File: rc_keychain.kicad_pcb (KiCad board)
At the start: 4 copper layers, 63 x 18 mm, 139 parts, among them J2 TYPE-C 16PIN 2MD(073), J3 Touch_Surface_Top, J4 Touch_Surface_Bottom, J5 5034801200, Q1 2N7002T, SW1 TS35CA, U1 SF32LB525UC6, U10 LIS3DH, U12 SN74AUP1G17, U13 ST25R3916B-AQET, U2 GD25Q256EWIGR, U3 TPS25200DRVT, U4 USBLC6-2P6, U5 USBLC6-2P6, U6 CAP1208-1-A4-TR, U7 CAP1208-1-A4-TR, U8 DRV2603RUNT, U9 TPS61040DBV, Y1 48MHz, Y2 32.768khz, Y3 27.12MHz

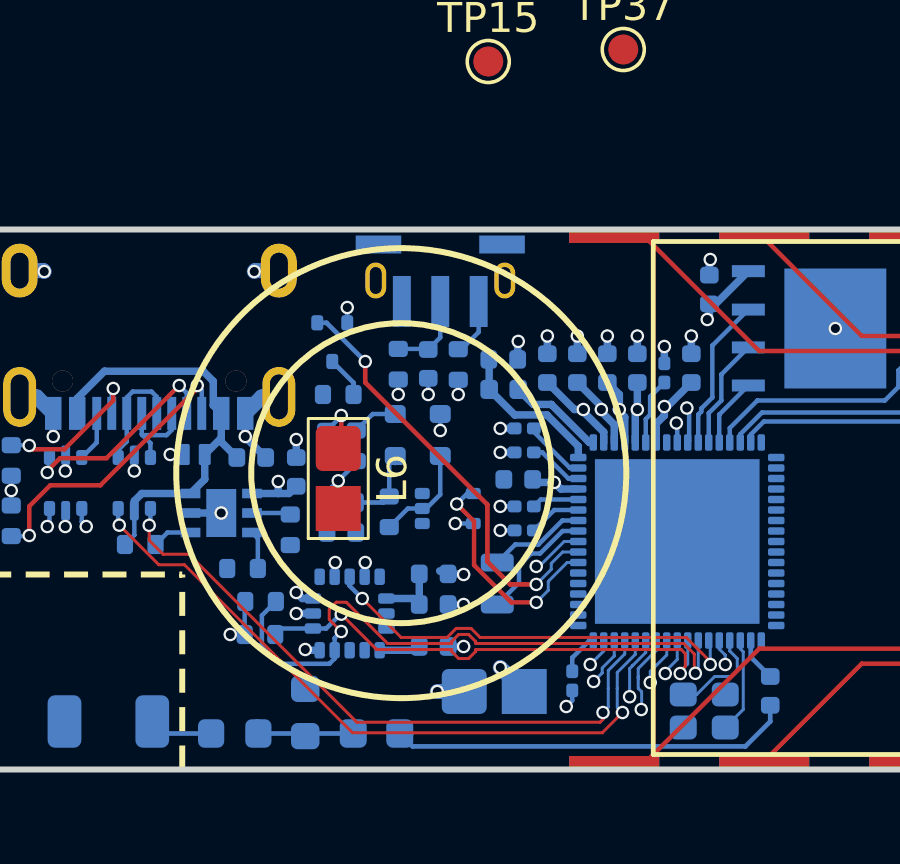
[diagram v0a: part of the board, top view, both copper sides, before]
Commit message: progress before stepping
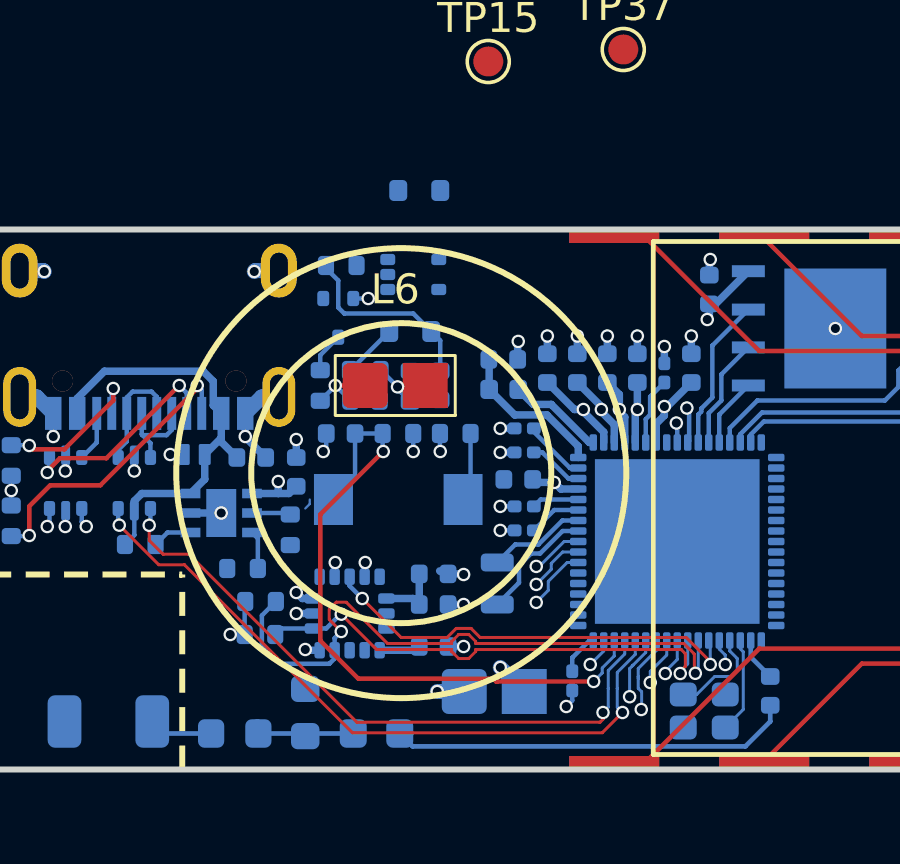
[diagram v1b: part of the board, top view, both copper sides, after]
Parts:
- SW1: value TS35CA -> HX 3X4X2-2P-1.6N; footprint TS35CA:KEY-SMD_TS35CA -> HX3x4x2-2P-1:KEY-SMD_L4.0-W3.0-LS4.9-1
- moved R21 8.36 mm to (51.8, 105.2), turned to 0 degrees
- moved D3 8.18 mm to (54.4, 102.7), turned to 180 degrees
- moved U12 7.88 mm to (54.2, 105.5)
- moved SW1 7.68 mm to (53.7, 113.0)
- moved C39 5.91 mm to (55.1, 109.2), turned to 90 degrees
- moved R22 4.52 mm to (54.1, 109.2), turned to -90 degrees
- moved C31 3.73 mm to (51.8, 110.8), turned to 180 degrees
- moved L6 3.64 mm to (53.6, 109.2), turned to 180 degrees
- moved D2 3.49 mm to (54.1, 107.4), turned to 180 degrees
- moved R20 2.53 mm to (52.6, 108.7), turned to 0 degrees
- moved R18 2.31 mm to (53.7, 110.8), turned to 0 degrees
- moved R17 2.30 mm to (55.6, 110.8), turned to 0 degrees
- moved C38 1.98 mm to (52.6, 109.7), turned to 0 degrees
- moved Q1 0.83 mm to (51.7, 106.9)
- moved R23 0.67 mm to (51.1, 109.2), turned to 90 degrees
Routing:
- net BUTTON: track 4.42 -> 22.6 mm, vias 1 -> 2
- net RFID_DAT: track 14.5 -> 1.96 mm, vias 2 -> 1
- net RFID_WAKE: track 7.69 -> 2.13 mm, vias 2 -> 1
- net Net-(D3-K): track 3.43 -> 0.00 mm
- net Net-(D2-K): track 4.01 -> 7.44 mm
- net GND: track 30.2 -> 29.5 mm, vias 38 -> 37
- net Net-(D2-A): track 4.60 -> 5.29 mm
- net VBUS: track 18.6 -> 18.0 mm
- net +3V3: track 10.4 -> 9.88 mm, vias 6 -> 5
